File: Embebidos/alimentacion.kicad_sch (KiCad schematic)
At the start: 18 parts, among them J2 Conn_01x02_Male, U3 SPX3819M5-L-3-3, U4 MIC29302WT, U5 MIC5219-3.3YM5

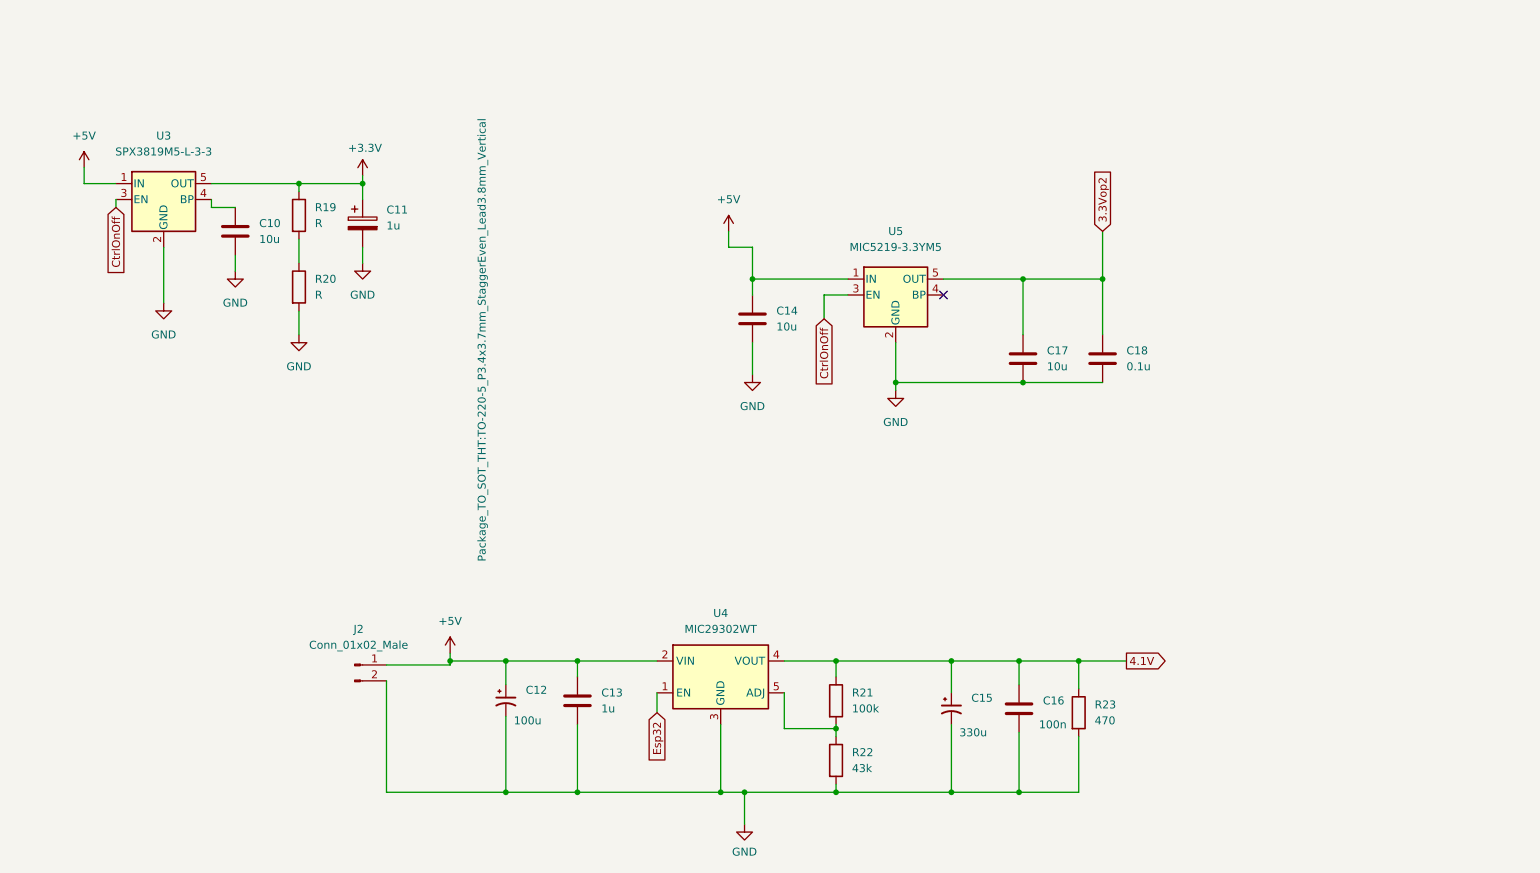
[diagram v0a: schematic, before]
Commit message: mejoras alimentacion
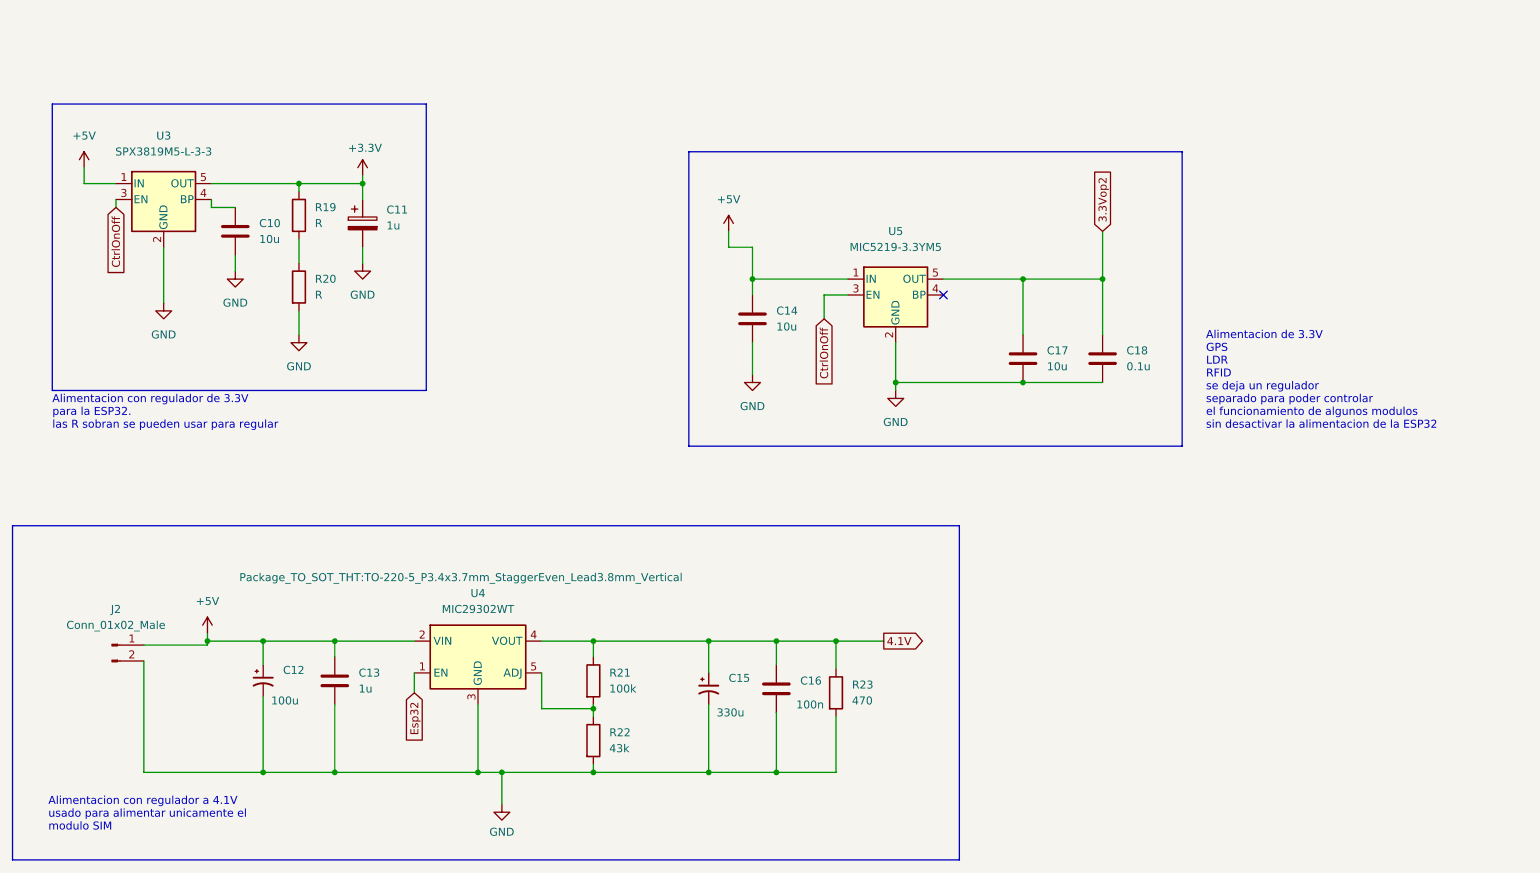
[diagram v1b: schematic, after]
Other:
- note added: "Alimentacion con regulador a 4.1V usado para alimentar unicamente el modulo SIM"
- note added: "Alimentacion con regulador de 3.3V para la ESP32. las R sobran se pueden usar para regular"
- note added: "Alimentacion de 3.3V GPS LDR RFID se deja un regulador separado para poder controlar el funcionamiento de algunos modulos sin desactivar la alimentacion de la ESP32"
- moved on the sheet: C12, C13, C15, C16, J2, R21, R22, R23, U4
